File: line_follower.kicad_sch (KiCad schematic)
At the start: 71 parts, among them J1 Conn_01x20_Socket, J10 Conn_01x20_Pin, J11 Conn_01x20_Pin, J2 Conn_01x20_Socket, J3 Conn_01x06_Socket, J4 Conn_01x06_Socket, J5 XT60-M, J6 Conn_01x02_Socket, J7 Conn_01x02_Socket, J8 Conn_01x06_Socket, J9 MOTOR OUTPUTS, SW1 SW_Push, SW2 SW_Push, SW3 SW_Push, SW4 SW_Push, SW5 SW_Push, SW6 SW_Push, SW7 SW_Push

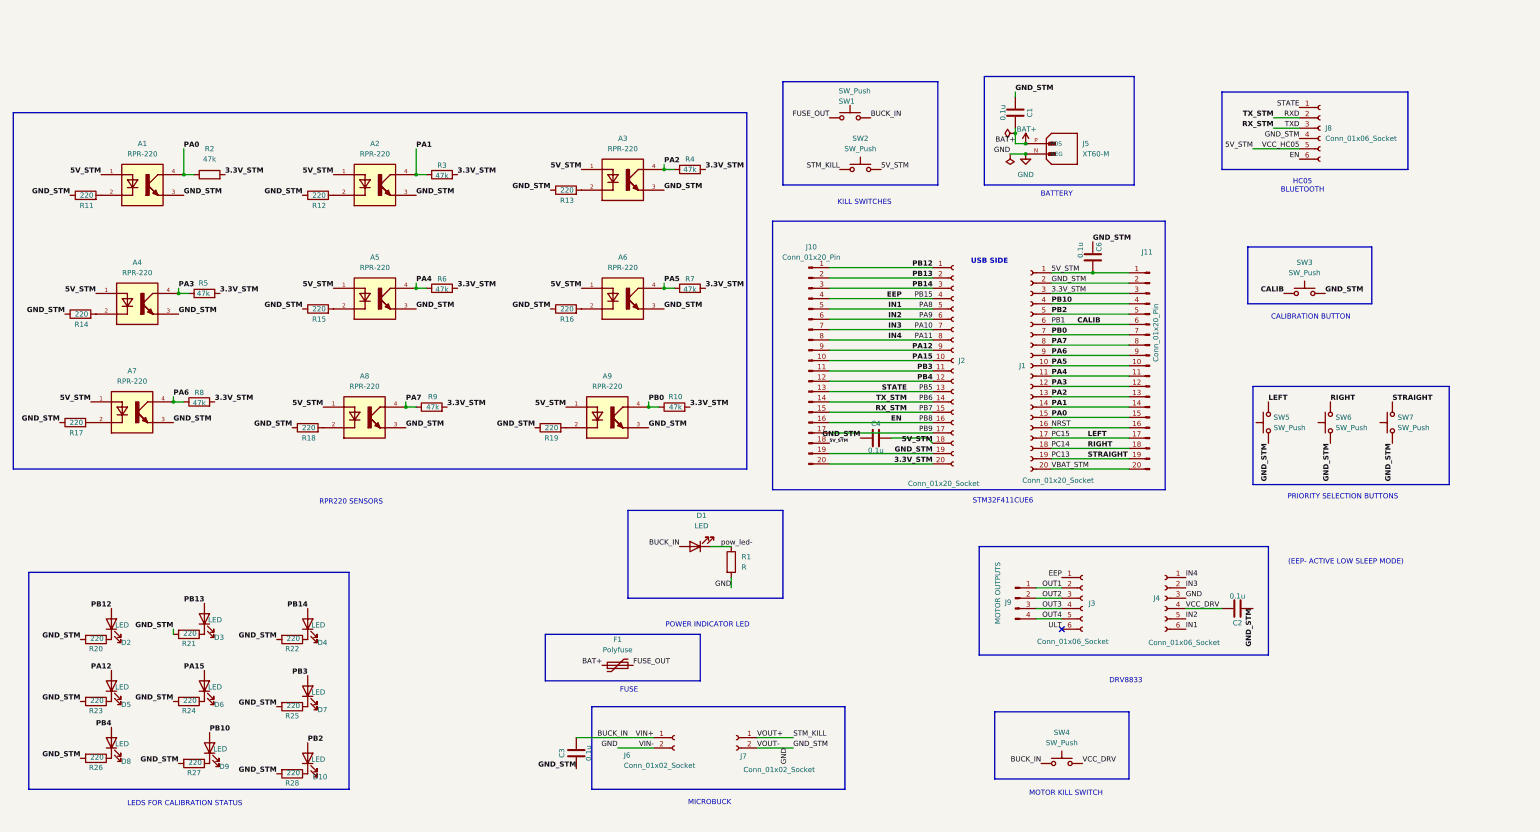
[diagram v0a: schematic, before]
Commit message: schematic updated by veena
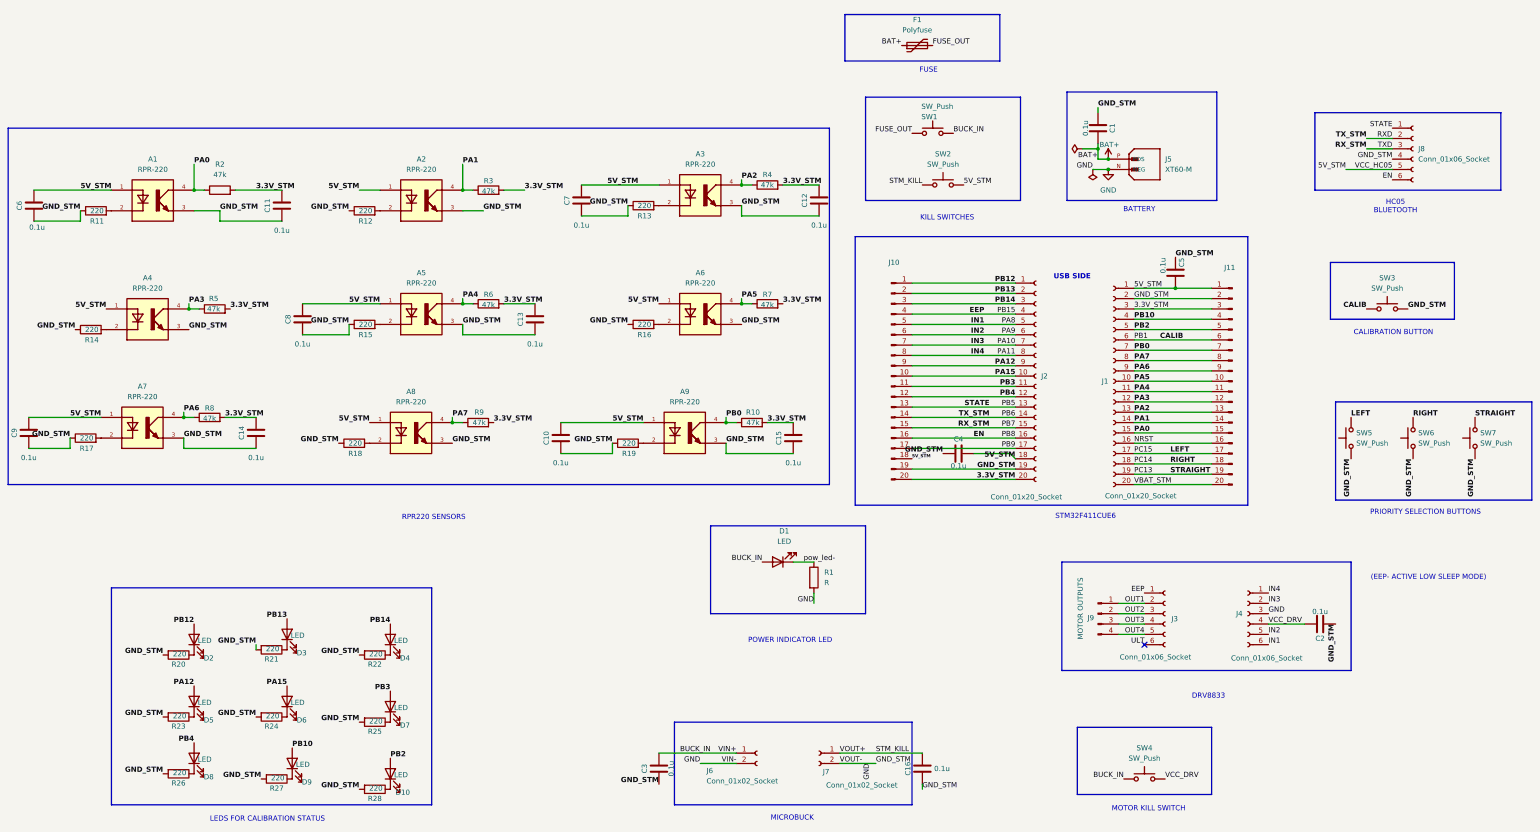
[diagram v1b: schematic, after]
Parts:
- added C10, C11, C12, C13, C14, C15, C16, C6, C7, C8, C9: 0.1u, symbol Device:C
- renumbered C6 to C5
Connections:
- net 3.3V_STM: now also C11.2, C12.2, C13.2, C14.2, C15.2
- net 5V_STM: now also C10.2, C6.2, C7.2, C8.2, C9.2
- net GND: now also C10.1, C11.1, C12.1, C13.1, C14.1, C15.1, C16.1, C6.1, C7.1, C8.1, C9.1
- net STM_KILL: now also C16.2
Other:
- moved on the sheet: A1, A2, A3, A4, A5, A6, A7, A8, A9, C1, C2, C3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

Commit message: minor changes
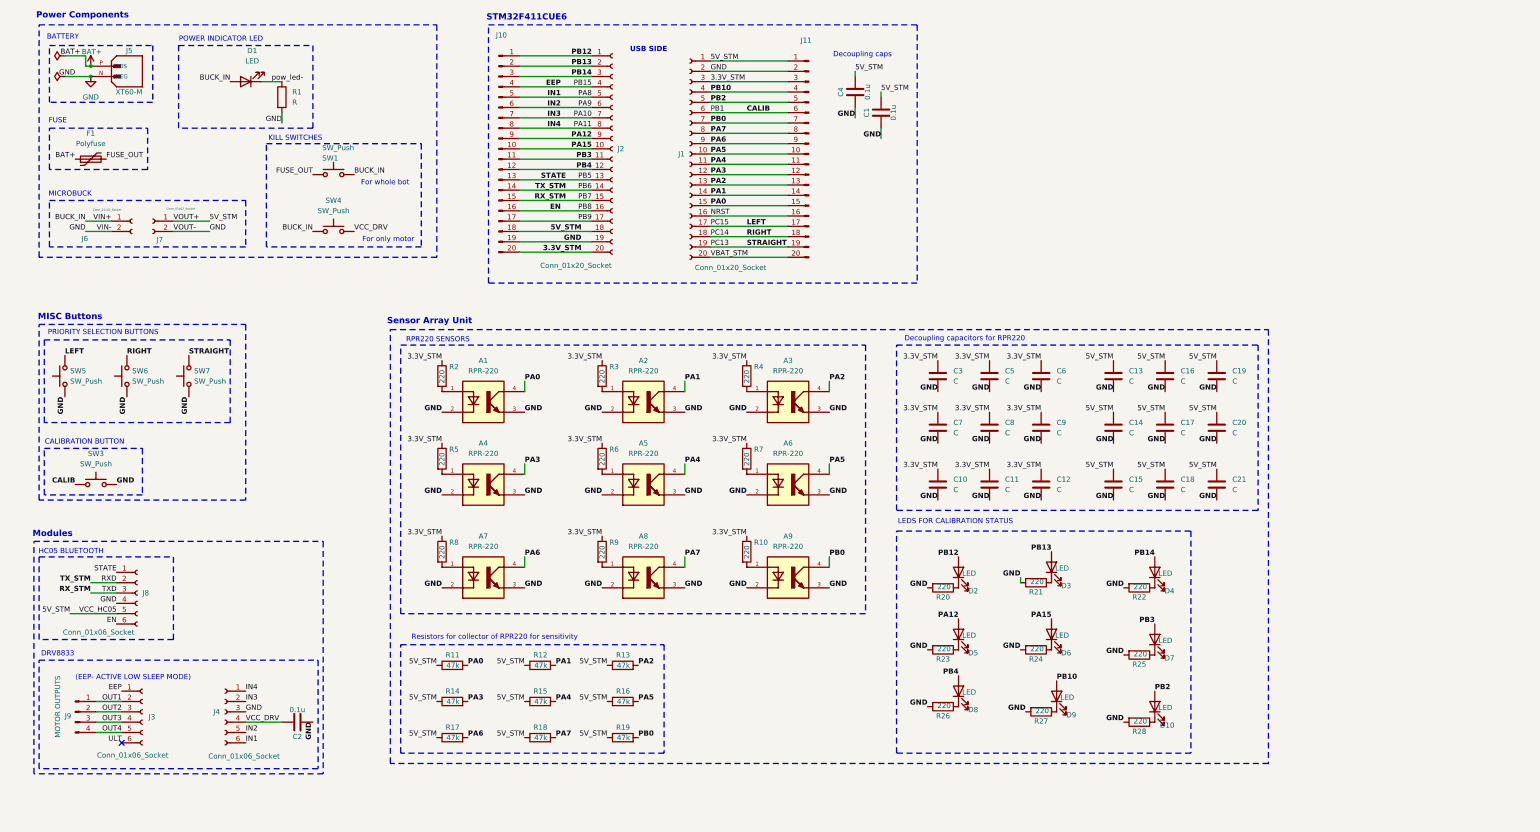
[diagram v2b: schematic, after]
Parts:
- removed SW2: SW_Push, symbol Switch:SW_Push
- added C17, C18, C19, C20, C21: C, symbol Device:C
- C10, C11, C12, C13, C14, C15, C16, C3, C5, C6, C7, C8, C9: value 0.1u -> C
- R10, R2, R3, R4, R5, R6, R7, R8, R9: value 47k -> 220
- R11, R12, R13, R14, R15, R16, R17, R18, R19: value 220 -> 47k
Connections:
- net 3.3V_STM: now also C10.1, C11.1, C12.1, C3.1, C5.1, C6.1, C7.1, C8.1, C9.1, R10.1, R2.1, R3.1, R4.1, R5.1, R6.1, R7.1, R8.1, R9.1; no longer C11.2, C12.2, C13.2, C14.2, C15.2, R10.2, R2.2, R3.2, R4.2, R5.2, R6.2, R7.2, R8.2, R9.2
- net 5V_STM: now also C1.2, C13.1, C14.1, C15.1, C16.1, J7.1 (Pin_1), R11.1, R12.1, R13.1, R14.1, R15.1, R16.1, R17.1, R18.1, R19.1, C17.1, C18.1, C19.1, C20.1, C21.1; no longer A1.1, A2.1, A3.1, A4.1, A5.1, A6.1, A7.1, A8.1, A9.1, C10.2, C5.2, C6.2, C7.2, C8.2, C9.2
- net BAT+: no longer C1.2
- net BUCK_IN: no longer C3.2
- net GND: now also A1.2, A2.2, A3.2, A4.2, A5.2, A6.2, A7.2, A8.2, A9.2, C10.2, C11.2, C12.2, C13.2, C14.2, C15.2, C16.2, C3.2, C5.2, C6.2, C7.2, C8.2, C9.2, C17.2, C18.2, C19.2, C20.2, C21.2; no longer C10.1, C11.1, C12.1, C13.1, C14.1, C15.1, C16.1, C3.1, C5.1, C6.1, C7.1, C8.1, C9.1, R11.1, R12.1, R13.1, R14.1, R15.1, R16.1, R17.1, R18.1, R19.1
- net PA0: now also R11.2; no longer R2.1
- net PA1: now also R12.2; no longer R3.1
- net PA2: now also R13.2; no longer R4.1
- net PA3: now also R14.2; no longer R5.1
- net PA4: now also R15.2; no longer R6.1
- net PA5: now also R16.2; no longer R7.1
- net PA6: now also R17.2; no longer R8.1
- net PA7: now also R18.2; no longer R9.1
- net PB0: now also R19.2; no longer R10.1
- removed net STM_KILL: C16.2, J7.1 (Pin_1)
- new net: A2.1, R3.2
- new net: A8.1, R9.2
- new net: A1.1, R2.2
- new net: A6.1, R7.2
- new net: A7.1, R8.2
- new net: A4.1, R5.2
- new net: A5.1, R6.2
- new net: A3.1, R4.2
- new net: A9.1, R10.2
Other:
- note added: "Decoupling capacitors for RPR220"
- note added: "Decoupling caps"
- note added: "For only motor"
- note added: "For whole bot"
- note added: "MISC Buttons"
- note added: "Modules"
- note added: "Power Components"
- note added: "Resistors for collector of RPR220 for sensitivity"
- note added: "Sensor Array Unit"
- note removed: "MOTOR KILL SWITCH"
- moved on the sheet: A1, A2, A3, A4, A5, A6, A7, A8, A9, C2, C4, D1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
